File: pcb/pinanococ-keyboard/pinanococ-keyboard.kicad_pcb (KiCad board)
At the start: 2 copper layers, 146.5 x 137.2 mm, 70 parts, among them J1 AudioJack4, SW1 SW_Push, SW10 SW_Push, SW11 SW_Push, SW12 SW_Push, SW14 SW_Push, SW15 SW_Push, SW16 SW_Push, SW17 SW_Push, SW18 SW_Push, SW2 SW_Push, SW20 SW_Push_Dual_x2, SW21 SW_Push, SW22 SW_Push, SW23 SW_Push, SW24 SW_Push, SW26 SW_Push_Dual_x2, SW27 SW_Push, SW28 SW_Push, SW29 SW_Push, SW3 SW_Push, SW30 SW_Push, SW32 SW_Push_Dual_x2, SW33 SW_Push, SW34 SW_Push, SW35 SW_Push, SW36 SW_Push, SW37 SW_Push, SW38 Rotary_Encoder_Switch, SW4 SW_Push, SW5 SW_Push, SW6 SW_Push, SW8 SW_Push, SW9 SW_Push, U1 Pico

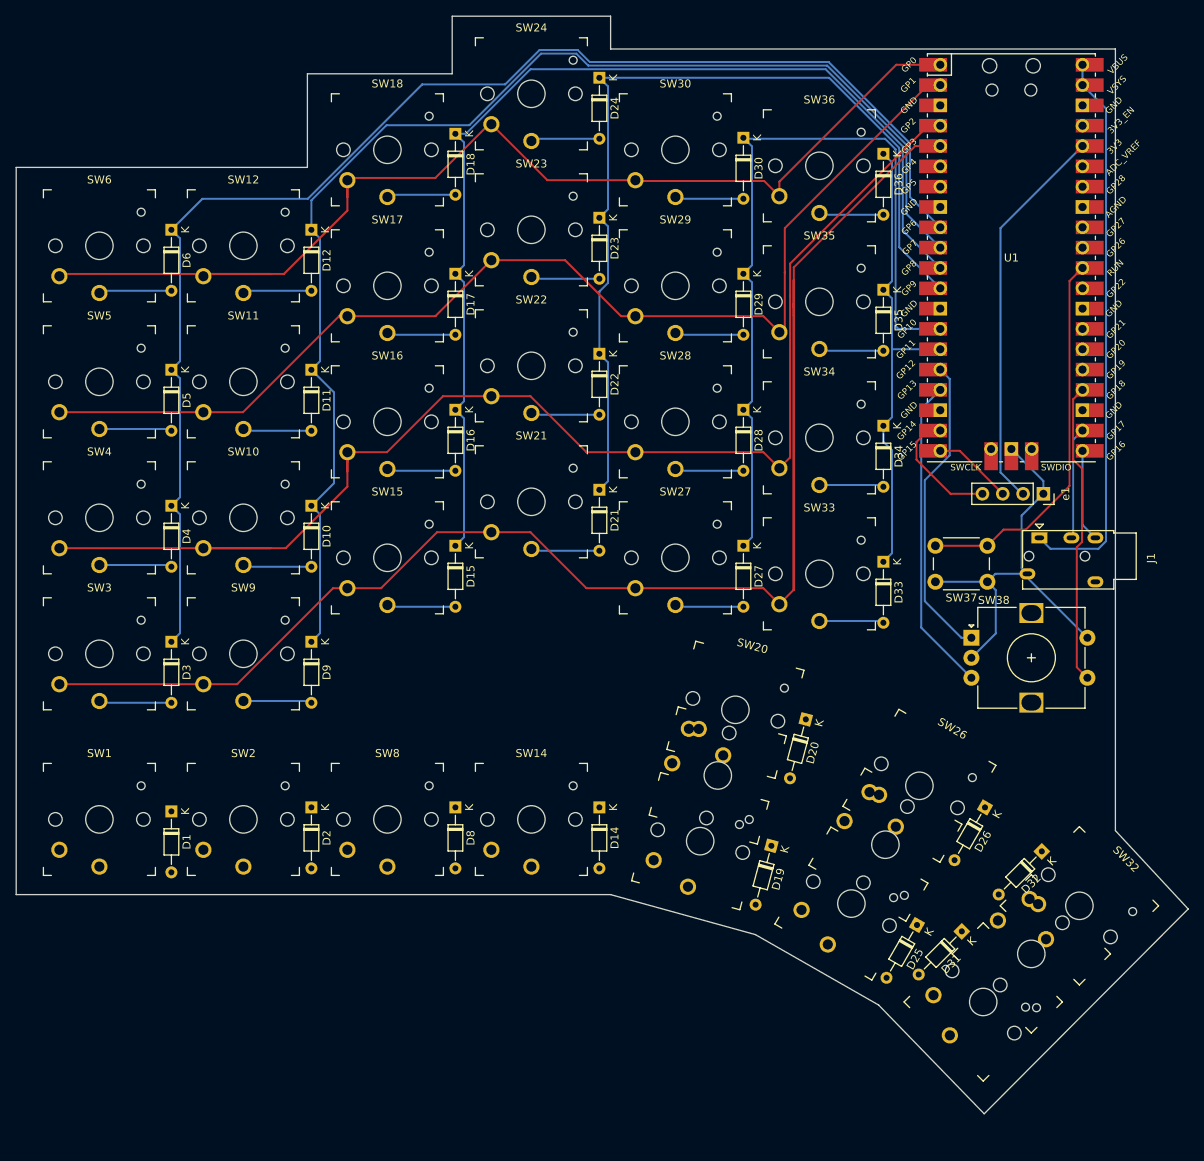
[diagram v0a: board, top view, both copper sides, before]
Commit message: pcb component layout
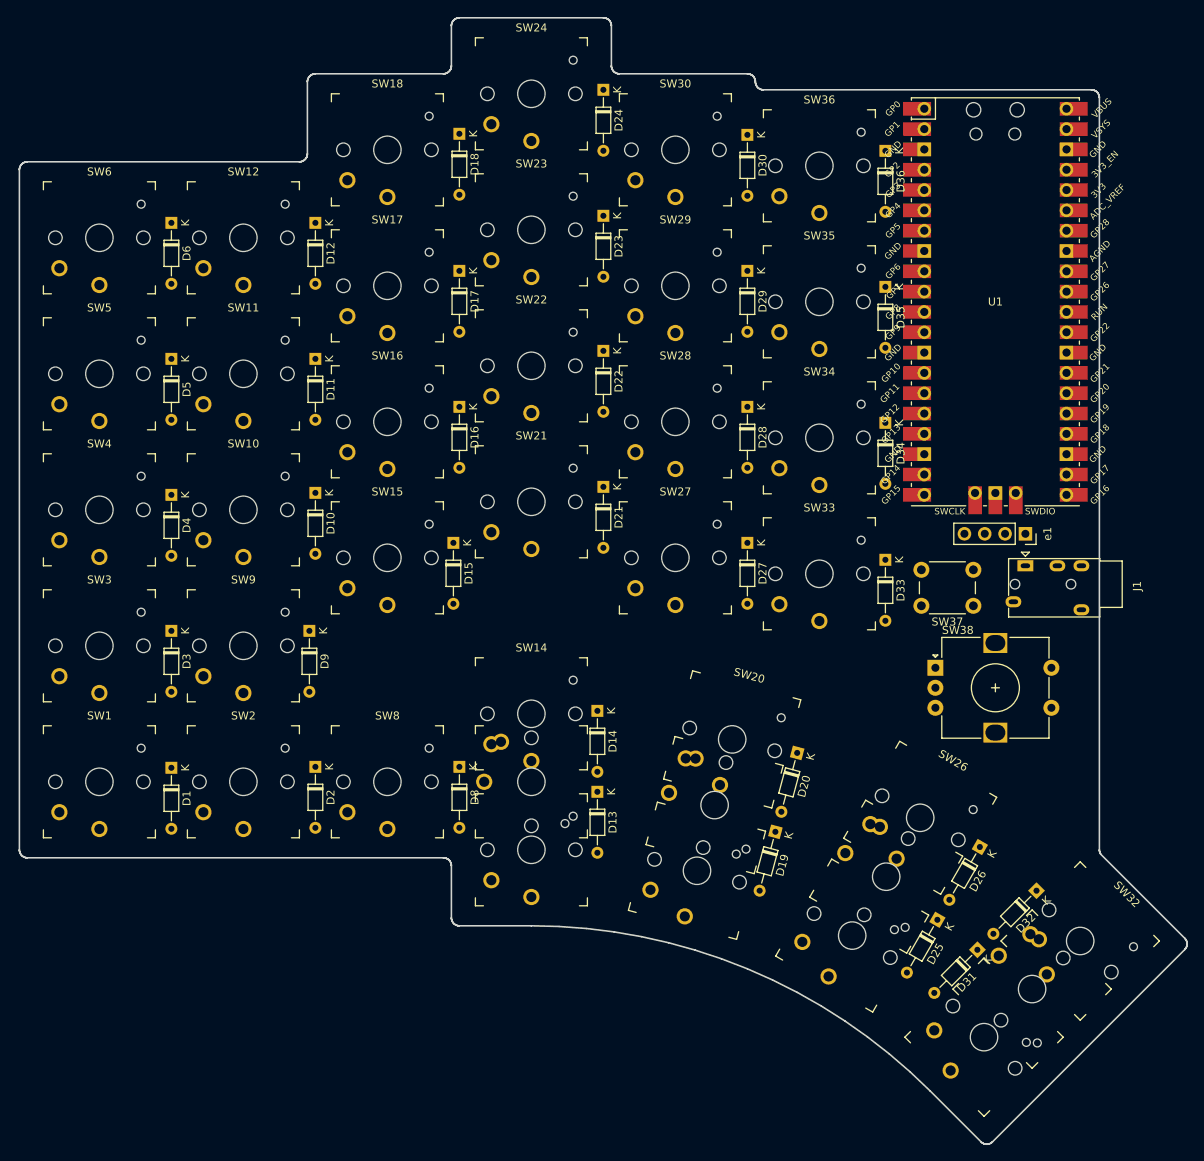
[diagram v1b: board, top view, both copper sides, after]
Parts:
- added D13: D_ALT, Diode_THT:D_DO-34_SOD68_P7.62mm_Horizontal, F.Cu at (86.2, 134.2)
- SW14: value SW_Push -> SW_Push_Dual_x2; footprint keyswitches:SW_PG1350 -> keyswitches:SW_PG1350_double_rotate
- moved SW14 13.2 mm to (78.0, 124.5)
- moved D14 12.1 mm to (86.2, 124.1)
- moved SW38 5.86 mm to (128.5, 118.8)
- moved U1 5.85 mm to (136.0, 73.0)
- moved e1 5.48 mm to (139.8, 102.0)
- moved D1 5.45 mm to (33.0, 131.2)
- moved D2 5.09 mm to (51.0, 131.1)
- moved D8 5.09 mm to (69.0, 131.1)
- moved D26 4.99 mm to (134.1, 141.2)
- moved D32 4.96 mm to (141.1, 146.6)
- moved SW1 4.70 mm to (24.0, 133.0)
- moved SW2 4.70 mm to (42.0, 133.0)
- moved SW8 4.70 mm to (60.0, 133.0)
- moved SW32 4.40 mm to (146.6, 152.9)
- moved D20 4.33 mm to (111.2, 129.4)
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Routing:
- net ROW_2: track 214.2 -> 0.00 mm
- net COL_0: track 172.7 -> 0.00 mm
- net ROW_3: track 167.2 -> 0.00 mm
- net COL_1: track 160.6 -> 0.00 mm
- net ROW_5: track 142.8 -> 0.00 mm
- net ROW_4: track 141.7 -> 0.00 mm
- net COL_2: track 134.6 -> 0.00 mm
- net COL_3: track 115.0 -> 0.00 mm
- net COL_4: track 101.4 -> 0.00 mm
- net VBUS: track 70.1 -> 0.00 mm
- net COL_5: track 59.7 -> 0.00 mm
- net GND: track 52.9 -> 0.00 mm
- net +3V3: track 49.0 -> 0.00 mm
- net Reset: track 47.8 -> 0.00 mm
- net ROT_B: track 39.6 -> 0.00 mm
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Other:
- board size 146.5 x 137.2 mm -> 146 x 140.8 mm
- net class Default: clearance 0.2 -> 0.254
- rule trace_clearance: 0.2 -> 0.254
